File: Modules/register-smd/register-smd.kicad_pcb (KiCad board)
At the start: 2 copper layers, 48.8 x 22.1 mm, 30 parts, among them J8 Conn_01x14, U1 74HC273, U2 74HC08, U47 74HC245

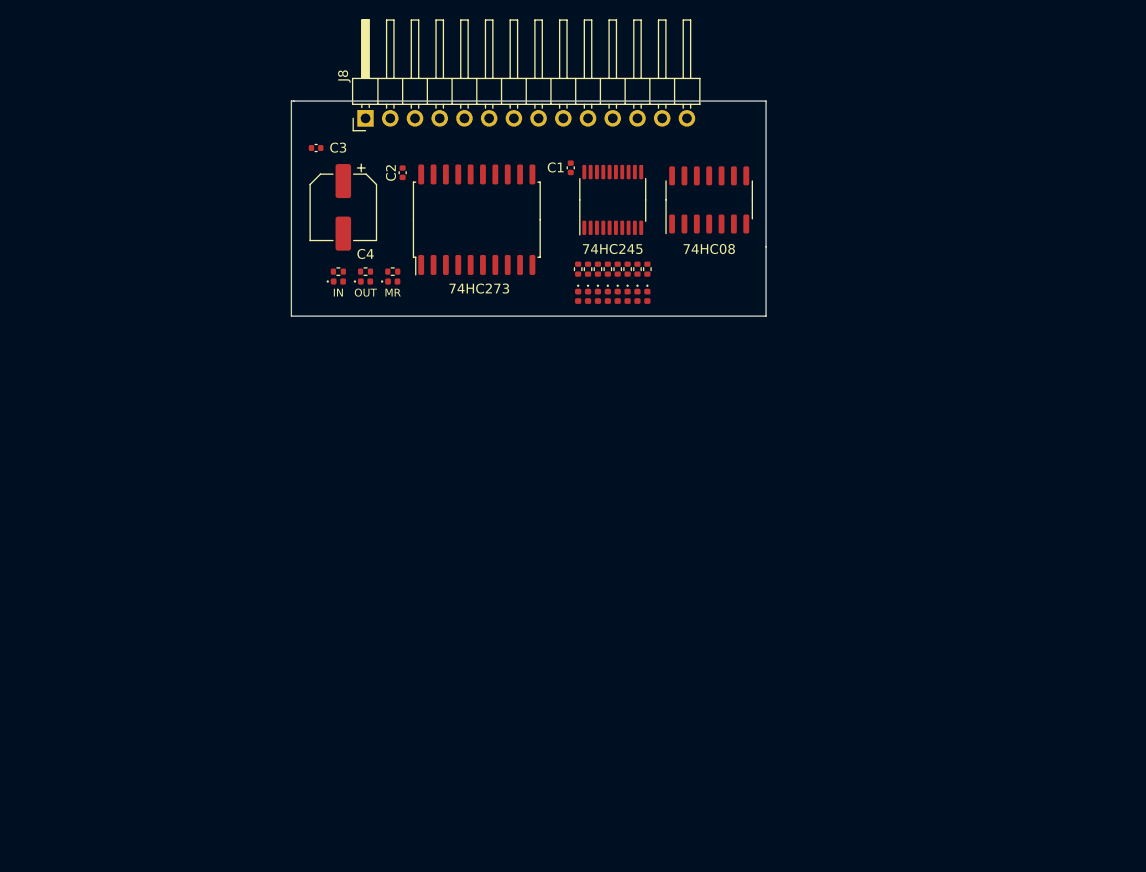
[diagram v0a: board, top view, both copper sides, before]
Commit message: Saving
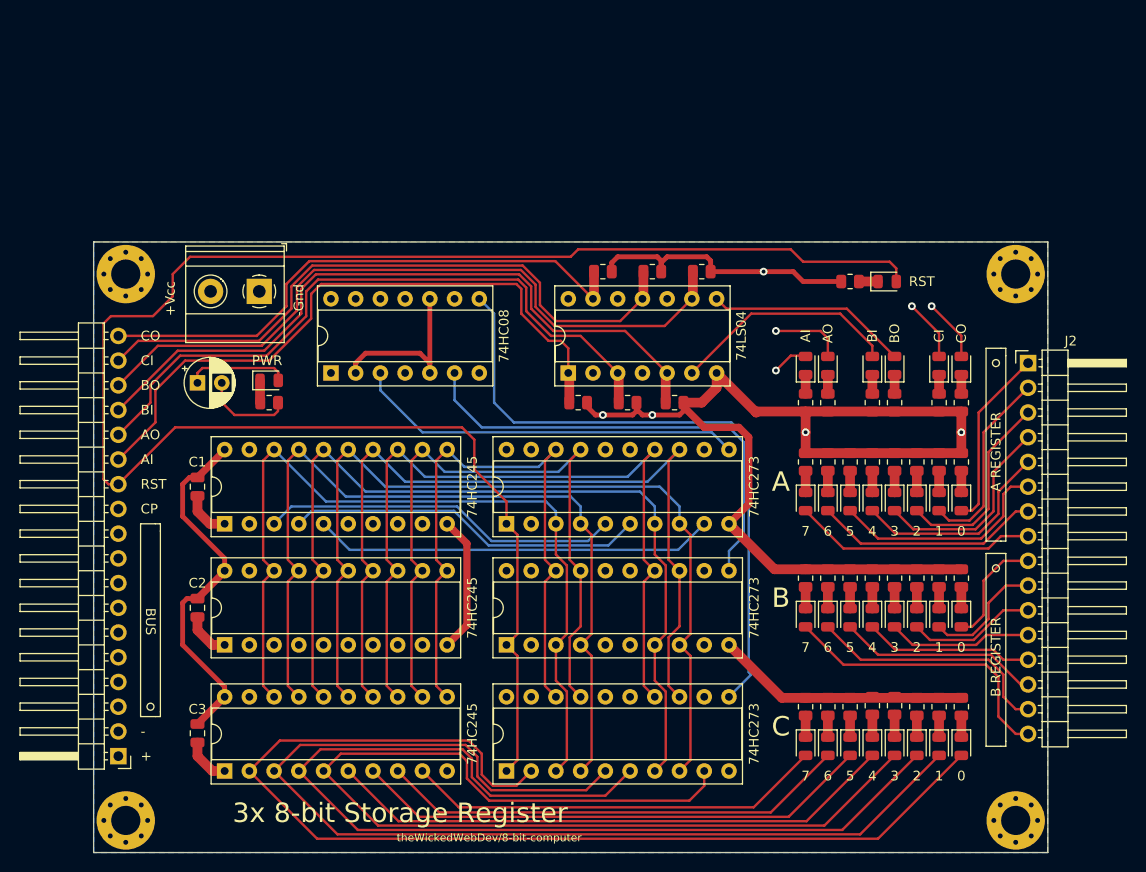
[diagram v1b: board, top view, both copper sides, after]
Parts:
- added D12: LED, LED_SMD:LED_0805_2012Metric, F.Cu at (141.7, 85.1)
- added D13: LED, LED_SMD:LED_0805_2012Metric, F.Cu at (139.4, 85.1)
- added D14: LED, LED_SMD:LED_0805_2012Metric, F.Cu at (137.2, 85.1)
- added D15: LED, LED_SMD:LED_0805_2012Metric, F.Cu at (134.9, 85.1)
- added D16: LED, LED_SMD:LED_0805_2012Metric, F.Cu at (132.6, 85.1)
- added D17: LED, LED_SMD:LED_0805_2012Metric, F.Cu at (130.3, 85.1)
- added D18: LED, LED_SMD:LED_0805_2012Metric, F.Cu at (128.0, 85.1)
- added D19: LED, LED_SMD:LED_0805_2012Metric, F.Cu at (125.7, 85.1)
- added D20: LED, LED_SMD:LED_0805_2012Metric, F.Cu at (132.6, 59.2)
- added D21: LED, LED_SMD:LED_0805_2012Metric, F.Cu at (134.9, 59.2)
- added D22: LED, LED_SMD:LED_0805_2012Metric, F.Cu at (141.7, 98.3)
- added D23: LED, LED_SMD:LED_0805_2012Metric, F.Cu at (139.4, 98.3)
- added D24: LED, LED_SMD:LED_0805_2012Metric, F.Cu at (137.2, 98.3)
- added D25: LED, LED_SMD:LED_0805_2012Metric, F.Cu at (134.9, 98.3)
- added D26: LED, LED_SMD:LED_0805_2012Metric, F.Cu at (132.6, 98.3)
- added D27: LED, LED_SMD:LED_0805_2012Metric, F.Cu at (130.3, 98.3)
- added D28: LED, LED_SMD:LED_0805_2012Metric, F.Cu at (128.0, 98.3)
- added D29: LED, LED_SMD:LED_0805_2012Metric, F.Cu at (125.7, 98.3)
- added D30: LED, LED_SMD:LED_0805_2012Metric, F.Cu at (139.4, 59.2)
- added D31: LED, LED_SMD:LED_0805_2012Metric, F.Cu at (141.7, 59.2)
- added D32: LED, LED_SMD:LED_0805_2012Metric, F.Cu at (70.6, 60.7)
- added J1: Screw_Terminal_01x02, TerminalBlock_Phoenix:TerminalBlock_Phoenix_MKDS-1,5-2_1x02_P5.00mm_Horizontal, F.Cu at (69.6, 51.6)
- added J2: Conn_01x16, Connector_PinHeader_2.54mm:PinHeader_1x16_P2.54mm_Horizontal, F.Cu at (148.6, 58.9)
- added R12: R_Small_US, Resistor_SMD:R_0805_2012Metric, F.Cu at (141.7, 81.0)
- added R13: R_Small_US, Resistor_SMD:R_0805_2012Metric, F.Cu at (139.4, 81.0)
- added R14: R_Small_US, Resistor_SMD:R_0805_2012Metric, F.Cu at (137.2, 81.0)
- added R15: R_Small_US, Resistor_SMD:R_0805_2012Metric, F.Cu at (134.9, 81.0)
- added R16: R_Small_US, Resistor_SMD:R_0805_2012Metric, F.Cu at (132.6, 81.0)
- added R17: R_Small_US, Resistor_SMD:R_0805_2012Metric, F.Cu at (130.3, 81.0)
- added R18: R_Small_US, Resistor_SMD:R_0805_2012Metric, F.Cu at (128.0, 81.0)
- added R19: R_Small_US, Resistor_SMD:R_0805_2012Metric, F.Cu at (125.7, 81.0)
- added R20: R_Small_US, Resistor_SMD:R_0805_2012Metric, F.Cu at (132.6, 63.0)
- added R21: R_Small_US, Resistor_SMD:R_0805_2012Metric, F.Cu at (134.9, 63.0)
- added R22: R_Small_US, Resistor_SMD:R_0805_2012Metric, F.Cu at (141.7, 94.2)
- added R23: R_Small_US, Resistor_SMD:R_0805_2012Metric, F.Cu at (139.4, 94.2)
- added R24: R_Small_US, Resistor_SMD:R_0805_2012Metric, F.Cu at (137.2, 94.2)
- added R25: R_Small_US, Resistor_SMD:R_0805_2012Metric, F.Cu at (134.9, 94.1)
- added R26: R_Small_US, Resistor_SMD:R_0805_2012Metric, F.Cu at (132.6, 94.1)
- added R27: R_Small_US, Resistor_SMD:R_0805_2012Metric, F.Cu at (130.3, 94.2)
- added R28: R_Small_US, Resistor_SMD:R_0805_2012Metric, F.Cu at (128.0, 94.2)
- added R29: R_Small_US, Resistor_SMD:R_0805_2012Metric, F.Cu at (125.7, 94.2)
- added R30: R_Small_US, Resistor_SMD:R_0805_2012Metric, F.Cu at (139.4, 63.0)
- added R31: R_Small_US, Resistor_SMD:R_0805_2012Metric, F.Cu at (141.7, 63.0)
- added R32: R_Small_US, Resistor_SMD:R_0805_2012Metric, F.Cu at (102.4, 63.0)
- added R33: R_Small_US, Resistor_SMD:R_0805_2012Metric, F.Cu at (107.4, 63.0)
- added R34: R_Small_US, Resistor_SMD:R_0805_2012Metric, F.Cu at (112.3, 63.0)
- added R35: R_Small_US, Resistor_SMD:R_0805_2012Metric, F.Cu at (115.1, 49.5)
- added R36: R_Small_US, Resistor_SMD:R_0805_2012Metric, F.Cu at (110.0, 49.5)
- added R37: R_Small_US, Resistor_SMD:R_0805_2012Metric, F.Cu at (104.9, 49.5)
- added R38: R_Small_US, Resistor_SMD:R_0805_2012Metric, F.Cu at (70.6, 63.0)
- added REF**: MountingHole_3mm_Pad_Via, MountingHole:MountingHole_3mm_Pad_Via, F.Cu at (147.3, 105.9)
- added REF**: MountingHole_3mm_Pad_Via, MountingHole:MountingHole_3mm_Pad_Via, F.Cu at (147.3, 49.8)
- added REF**: MountingHole_3mm_Pad_Via, MountingHole:MountingHole_3mm_Pad_Via, F.Cu at (55.9, 105.9)
- added REF**: MountingHole_3mm_Pad_Via, MountingHole:MountingHole_3mm_Pad_Via, F.Cu at (55.9, 49.8)
- added U3: 74HC273, Package_DIP:DIP-20_W7.62mm_Socket, F.Cu at (95.0, 87.9)
- added U4: 74LS04, Package_DIP:DIP-14_W7.62mm_Socket, F.Cu at (101.3, 59.9)
- added U5: 74HC245, Package_DIP:DIP-20_W7.62mm_Socket, F.Cu at (66.0, 87.9)
- added U6: 74HC273, Package_DIP:DIP-20_W7.62mm_Socket, F.Cu at (95.0, 100.8)
- added U7: 74HC245, Package_DIP:DIP-20_W7.62mm_Socket, F.Cu at (66.0, 100.8)
- C1, C2, C3: footprint Capacitor_SMD:C_0402_1005Metric -> Capacitor_SMD:C_0805_2012Metric
- C4: footprint Capacitor_SMD:CP_Elec_6.3x7.7 -> Capacitor_THT:CP_Radial_D5.0mm_P2.50mm
- D1, D2, D3, D4, D5, D6, D7, D8: footprint LED_SMD:LED_0402_1005Metric -> LED_SMD:LED_0805_2012Metric
- D10: value MR -> LED; footprint LED_SMD:LED_0402_1005Metric -> LED_SMD:LED_0805_2012Metric
- D11: value OUT -> LED; footprint LED_SMD:LED_0402_1005Metric -> LED_SMD:LED_0805_2012Metric
- D9: value IN -> LED; footprint LED_SMD:LED_0402_1005Metric -> LED_SMD:LED_0805_2012Metric
- J8: value Conn_01x14 -> Conn_01x18; footprint Connector_PinHeader_2.54mm:PinHeader_1x14_P2.54mm_Horizontal -> Connector_PinHeader_2.54mm:PinHeader_1x18_P2.54mm_Horizontal
- R1, R10, R11, R2, R3, R4, R5, R6, R7, R8, R9: footprint Resistor_SMD:R_0402_1005Metric -> Resistor_SMD:R_0805_2012Metric
- U1: footprint Package_SO:SOIC-20W_7.5x12.8mm_P1.27mm -> Package_DIP:DIP-20_W7.62mm_Socket
- U2: footprint Package_SO:SOIC-14_3.9x8.7mm_P1.27mm -> Package_DIP:DIP-14_W7.62mm_Socket
- U47: footprint Package_SO:TSSOP-20_4.4x6.5mm_P0.65mm -> Package_DIP:DIP-20_W7.62mm_Socket
- moved J8 70.3 mm to (55.1, 99.3), turned to 180 degrees
- moved C3 61.4 mm to (63.2, 97.0), turned to 270 degrees
- moved U47 51.9 mm to (66.0, 75.4)
- moved D10 50.8 mm to (134.1, 50.5)
- moved C1 50.4 mm to (63.2, 71.6), turned to 270 degrees
- moved R9 49.9 mm to (125.7, 63.0), turned to 270 degrees
- moved C2 49.4 mm to (63.2, 84.1), turned to 270 degrees
- moved R11 49.4 mm to (128.0, 63.0), turned to 270 degrees
- moved D9 48.8 mm to (125.7, 59.2), turned to 90 degrees
- moved D11 48.3 mm to (128.0, 59.2), turned to 90 degrees
- moved R10 47.0 mm to (130.3, 50.5), turned to 180 degrees
- moved U2 42.7 mm to (77.0, 59.9)
- moved D1 38.5 mm to (141.7, 73.2)
- moved R1 37.9 mm to (141.7, 69.1)
- moved D2 37.5 mm to (139.4, 73.2)
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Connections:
- D1 pad 2: /R0 -> /A0
- D11 pad 2: RO -> AO
- D2 pad 2: /R1 -> /A1
- D3 pad 2: /R2 -> /A2
- D4 pad 2: /R3 -> /A3
- D5 pad 2: /R4 -> /A4
- D6 pad 2: /R5 -> /A5
- D7 pad 2: /R6 -> /A6
- D8 pad 2: /R7 -> /A7
- D9 pad 2: RI -> AI
- J8 pad 1: GND -> VCC
- J8 pad 10: BUS_03 -> BUS_07
- J8 pad 11: BUS_04 -> CLOCK
- J8 pad 12: BUS_05 -> MR
- J8 pad 13: BUS_06 -> !AI
- J8 pad 14: BUS_07 -> !AO
- J8 pad 2: VCC -> GND
- J8 pad 3: CLOCK -> BUS_00
- J8 pad 4: RI -> BUS_01
- J8 pad 5: RO -> BUS_02
- J8 pad 6: MR -> BUS_03
- J8 pad 7: BUS_00 -> BUS_04
- J8 pad 8: BUS_01 -> BUS_05
- J8 pad 9: BUS_02 -> BUS_06
- U1 pad 12: /R4 -> /A4
- U1 pad 15: /R5 -> /A5
- U1 pad 16: /R6 -> /A6
- U1 pad 19: /R7 -> /A7
- U1 pad 2: /R0 -> /A0
- U1 pad 5: /R1 -> /A1
- U1 pad 6: /R2 -> /A2
- U1 pad 9: /R3 -> /A3
- U2 pad 1: RI -> AI
- U2 pad 10: (no net) -> CLOCK
- U2 pad 4: (no net) -> BI
- U2 pad 5: (no net) -> CLOCK
- U2 pad 6: (no net) -> Net-(U2-Pad6)
- U2 pad 8: (no net) -> Net-(U2-Pad8)
- U2 pad 9: (no net) -> CI
- U47 pad 19: RO -> AO
- U47 pad 2: /R7 -> /A0
- U47 pad 3: /R6 -> /A1
- U47 pad 4: /R5 -> /A2
- U47 pad 5: /R4 -> /A3
- U47 pad 6: /R3 -> /A4
- U47 pad 7: /R2 -> /A5
- U47 pad 8: /R1 -> /A6
- U47 pad 9: /R0 -> /A7
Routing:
- net GND: track 0.00 -> 207.6 mm, vias 0 -> 5
- net MR: track 0.00 -> 182.6 mm
- net BUS_03: track 0.00 -> 134.1 mm
- net BUS_02: track 0.00 -> 134.1 mm
- net BUS_04: track 0.00 -> 130.9 mm
- net BUS_01: track 0.00 -> 128.0 mm
- net BUS_05: track 0.00 -> 126.2 mm
- net BUS_00: track 0.00 -> 125.2 mm
- net CO: track 0.00 -> 116.4 mm, vias 0 -> 1
- net BUS_06: track 0.00 -> 116.4 mm
- net /C0: track 0.00 -> 113.7 mm
- net /C1: track 0.00 -> 113.5 mm
- net BUS_07: track 0.00 -> 111.6 mm
- net /A0: track 0.00 -> 111.2 mm
- net /C3: track 0.00 -> 109.0 mm
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- added copper zone on B.Cu, net GND
- added copper zone on In2.Cu, net VCC
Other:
- board size 48.8 x 22.1 mm -> 98 x 62.7 mm
- copper layers 2 -> 4
- board text added: "+"
- board text added: "+Vcc"
- board text added: "-"
- board text added: "-Gnd"
- board text added: "0"
- board text added: "1"
- board text added: "2"
- board text added: "3"
- board text added: "3x 8-bit Storage Register"
- board text added: "4"
- board text added: "5"
- board text added: "6"
- board text added: "7"
- board text added: "A"
- board text added: "A REGISTER"
- board text added: "AI"
- board text added: "AO"
- board text added: "B"
- board text added: "B REGISTER"
- board text added: "BI"
- board text added: "BO"
- board text added: "BUS"
- board text added: "C"
- board text added: "CI"
- board text added: "CO"
- board text added: "CP"
- board text added: "PWR"
- board text added: "RST"
- board text added: "theWickedWebDev/8-bit-computer"
